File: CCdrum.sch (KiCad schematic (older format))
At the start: 31 parts, among them J1 USB_B_μ, J2 Program, J3 MIDI_out, SW1 SW_Push, SW2 SW_Push, U1 MSP430G2533, U2 AMS1117-3.3, U3 74AUP1G17

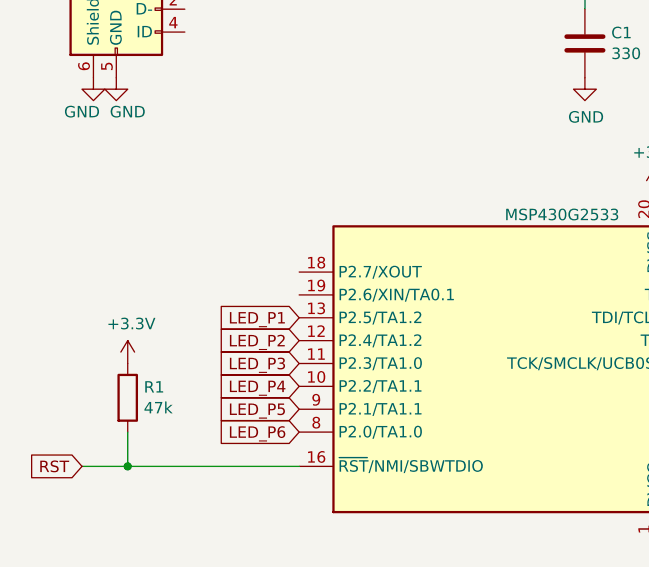
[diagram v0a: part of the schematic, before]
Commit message: PCB Routed
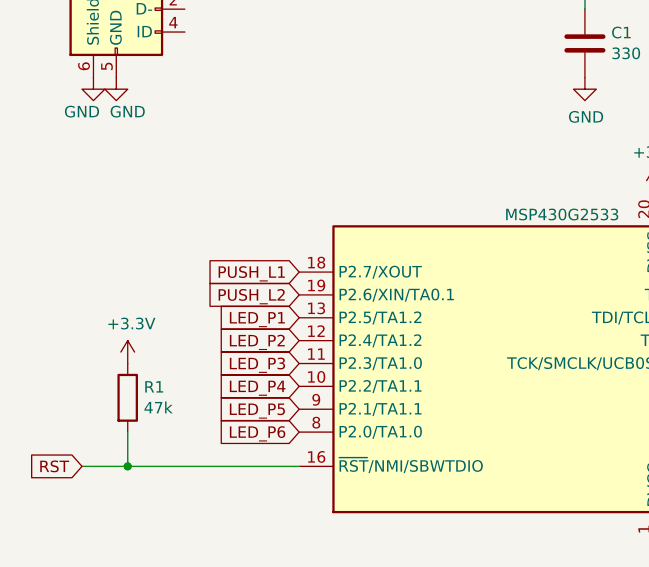
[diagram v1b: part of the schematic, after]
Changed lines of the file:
@@
 Text Notes 1500 6900 0    50   ~ 0
 they need some sort of visual feedback on the leds
+Text GLabel 2050 2450 0    50   Input ~ 0
+PUSH_L1
+Text GLabel 2050 2550 0    50   Input ~ 0
+PUSH_L2
 $EndSCHEMATC
